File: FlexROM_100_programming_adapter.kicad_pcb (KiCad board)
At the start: 2 copper layers, 18 x 35.8 mm, 2 parts, among them J1 LH535618 Socket, U1 28C256 pinout to programmer

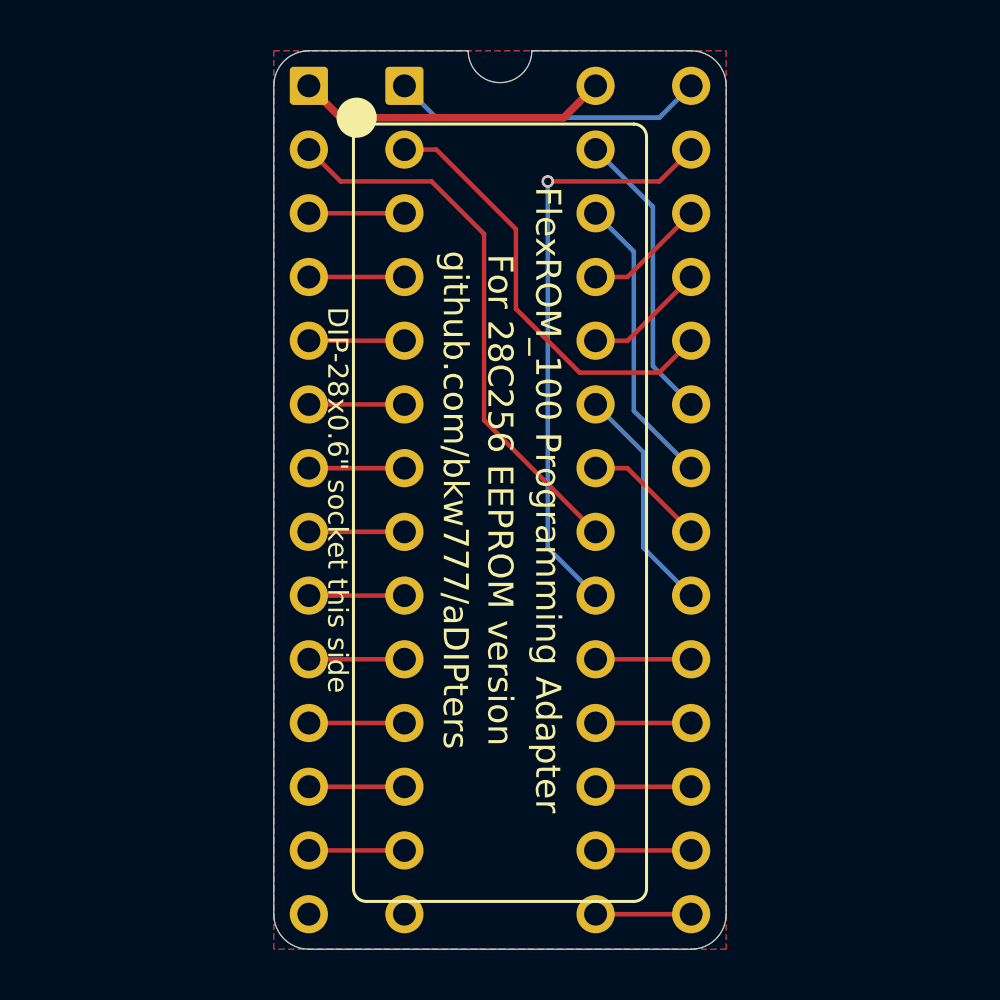
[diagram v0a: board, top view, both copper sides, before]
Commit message: various minor cleanups
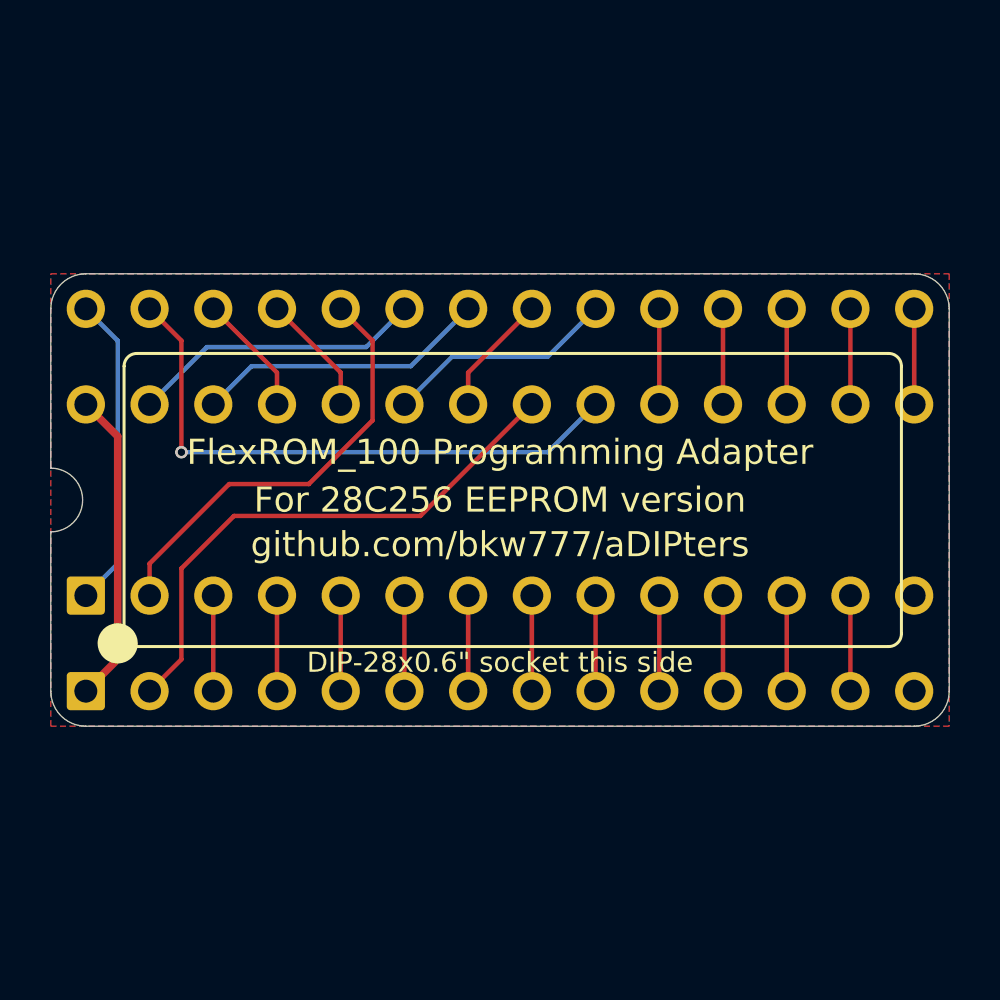
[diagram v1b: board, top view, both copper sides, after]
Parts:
- turned J1 to 90 degrees
- turned U1 to 90 degrees
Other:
- board size 18 x 35.8 mm -> 35.8 x 18 mm
